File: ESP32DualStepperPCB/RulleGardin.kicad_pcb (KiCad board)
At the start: 2 copper layers, 56 x 33 mm, 21 parts, among them J1 Power, J2 Prog, J3 Conn_01x05, U1 ESP32-S2-WROVER, U2 TSR_1-2433, U3 ULN2003A, U4 AZ1117-3.3

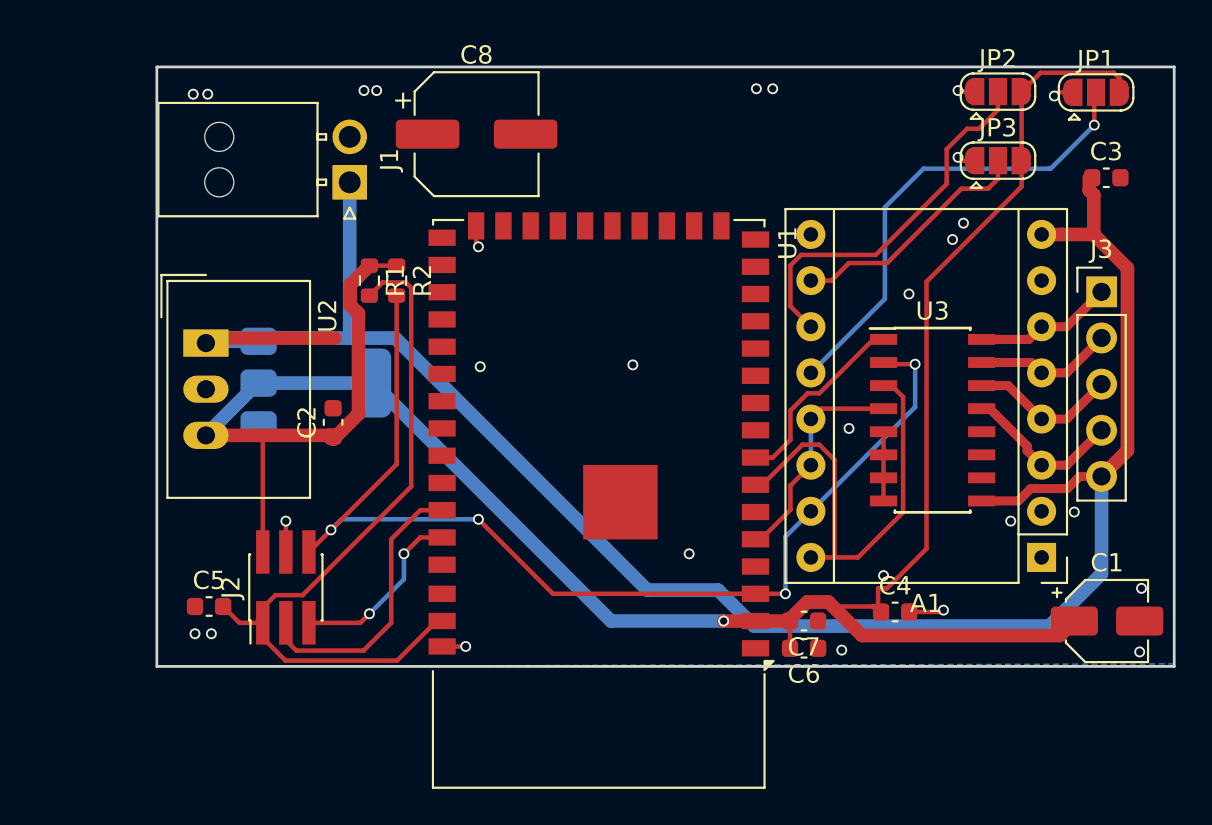
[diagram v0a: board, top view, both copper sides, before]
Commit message: updatePCB
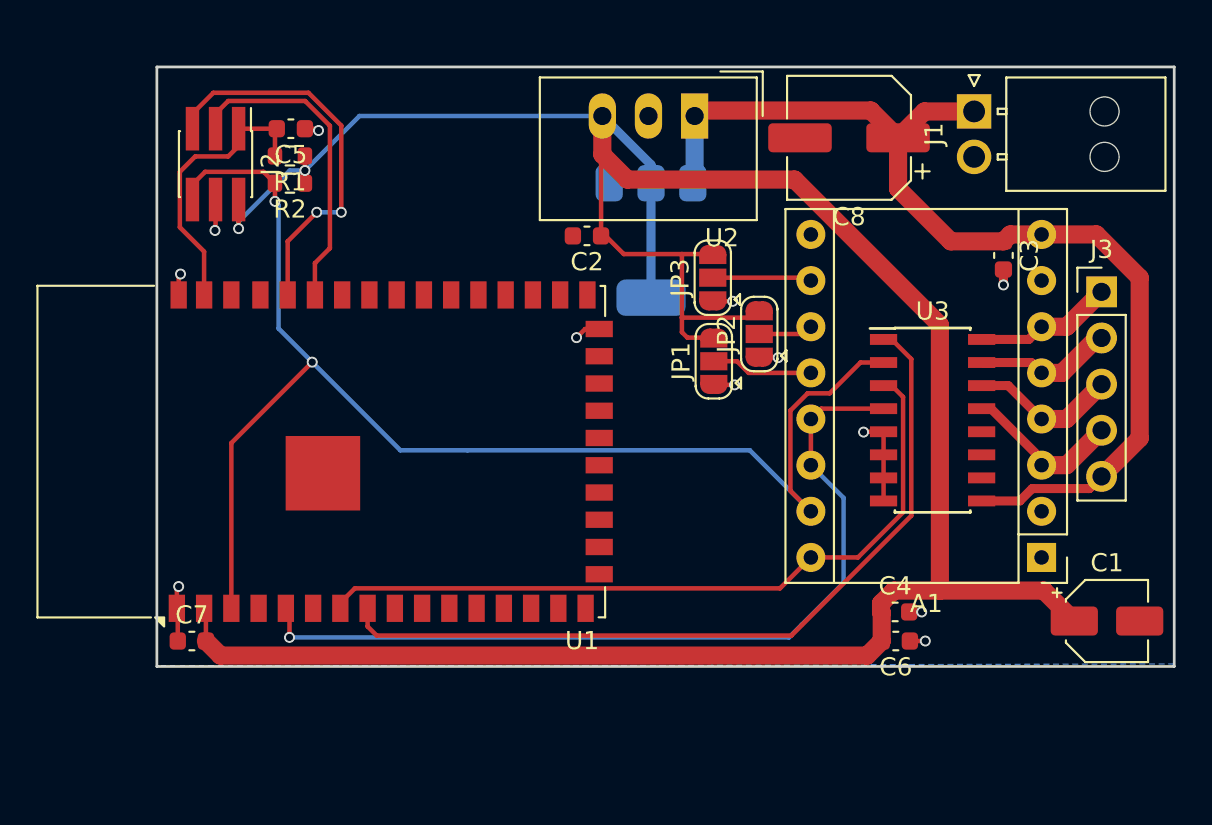
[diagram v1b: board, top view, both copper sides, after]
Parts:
- moved J1 34.6 mm to (193.0, 88.5), turned to -90 degrees
- moved C7 33.7 mm to (149.9, 117.6), turned to 0 degrees
- moved U2 29.7 mm to (177.6, 88.7), turned to 180 degrees
- moved C5 26.7 mm to (155.4, 89.4), turned to 180 degrees
- moved JP1 25.7 mm to (178.7, 102.2), turned to 90 degrees
- moved J2 23.6 mm to (151.2, 91.3), turned to -90 degrees
- moved C8 20.5 mm to (186.1, 89.9), turned to 180 degrees
- moved U4 20.1 mm to (175.2, 95.5), turned to -90 degrees
- moved JP2 18.7 mm to (181.2, 100.7), turned to 90 degrees
- moved C2 17.3 mm to (171.7, 95.3), turned to 180 degrees
- moved JP3 17.0 mm to (178.6, 97.6), turned to 90 degrees
- moved U1 11.5 mm to (160.9, 107.2), turned to 90 degrees
- moved R1 8.14 mm to (155.3, 90.9), turned to 180 degrees
- moved R2 7.95 mm to (155.3, 92.4), turned to 180 degrees
- moved C3 7.10 mm to (194.6, 96.4), turned to -90 degrees
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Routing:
- net +5V: track 109.2 -> 57.9 mm
- net /D2: track 12.3 -> 47.4 mm, vias 0 -> 1
- net /D5: track 10.7 -> 44.5 mm
- net EN: track 40.1 -> 15.7 mm
- net +3.3V: track 129.4 -> 153.5 mm, vias 1 -> 2
- net Net-(A1-M2): track 26.0 -> 5.61 mm, vias 1 -> 0
- net Net-(A1-M1): track 20.9 -> 3.01 mm
- net /D4: track 24.8 -> 41.0 mm
- net D0: track 60.4 -> 75.1 mm, vias 4 -> 2
- net RX: track 10.1 -> 21.6 mm
- net Net-(A1-M0): track 13.6 -> 5.47 mm
- net GND: track 12.8 -> 18.8 mm, vias 28 -> 12
- net TX: track 15.7 -> 17.6 mm
- net /Coil3: track 7.63 -> 8.25 mm
